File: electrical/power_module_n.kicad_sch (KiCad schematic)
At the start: 16 parts, among them J1 Ground connector from bulb wi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, J10 Need to cut return bulb wiring, J5 Power connector for bulb driv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, Q3 BC548B, Q5 IFRZ44N

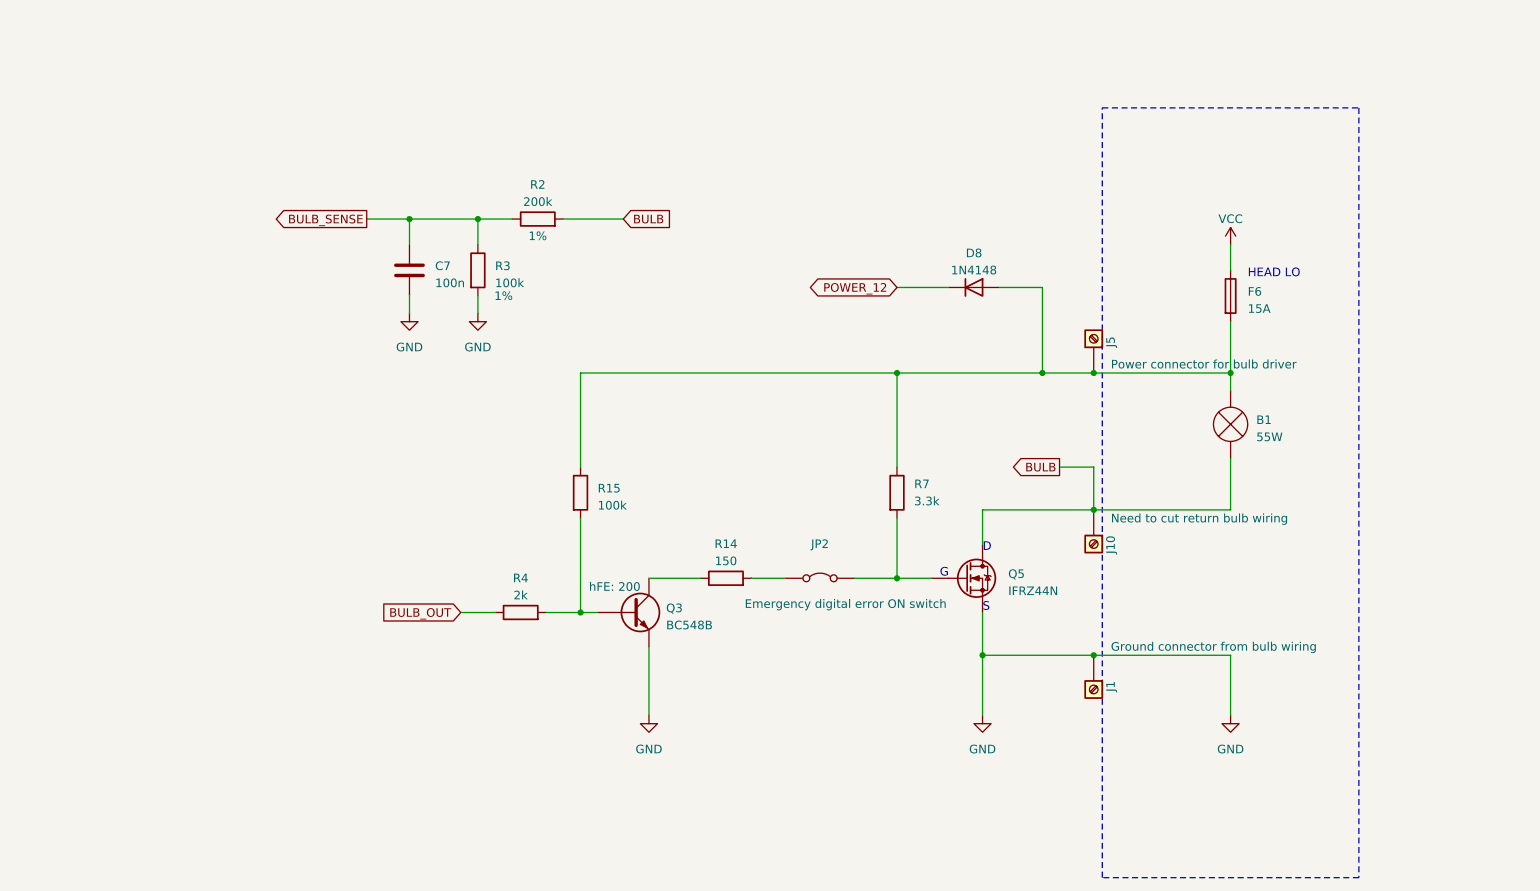
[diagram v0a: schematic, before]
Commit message: Względenie działa
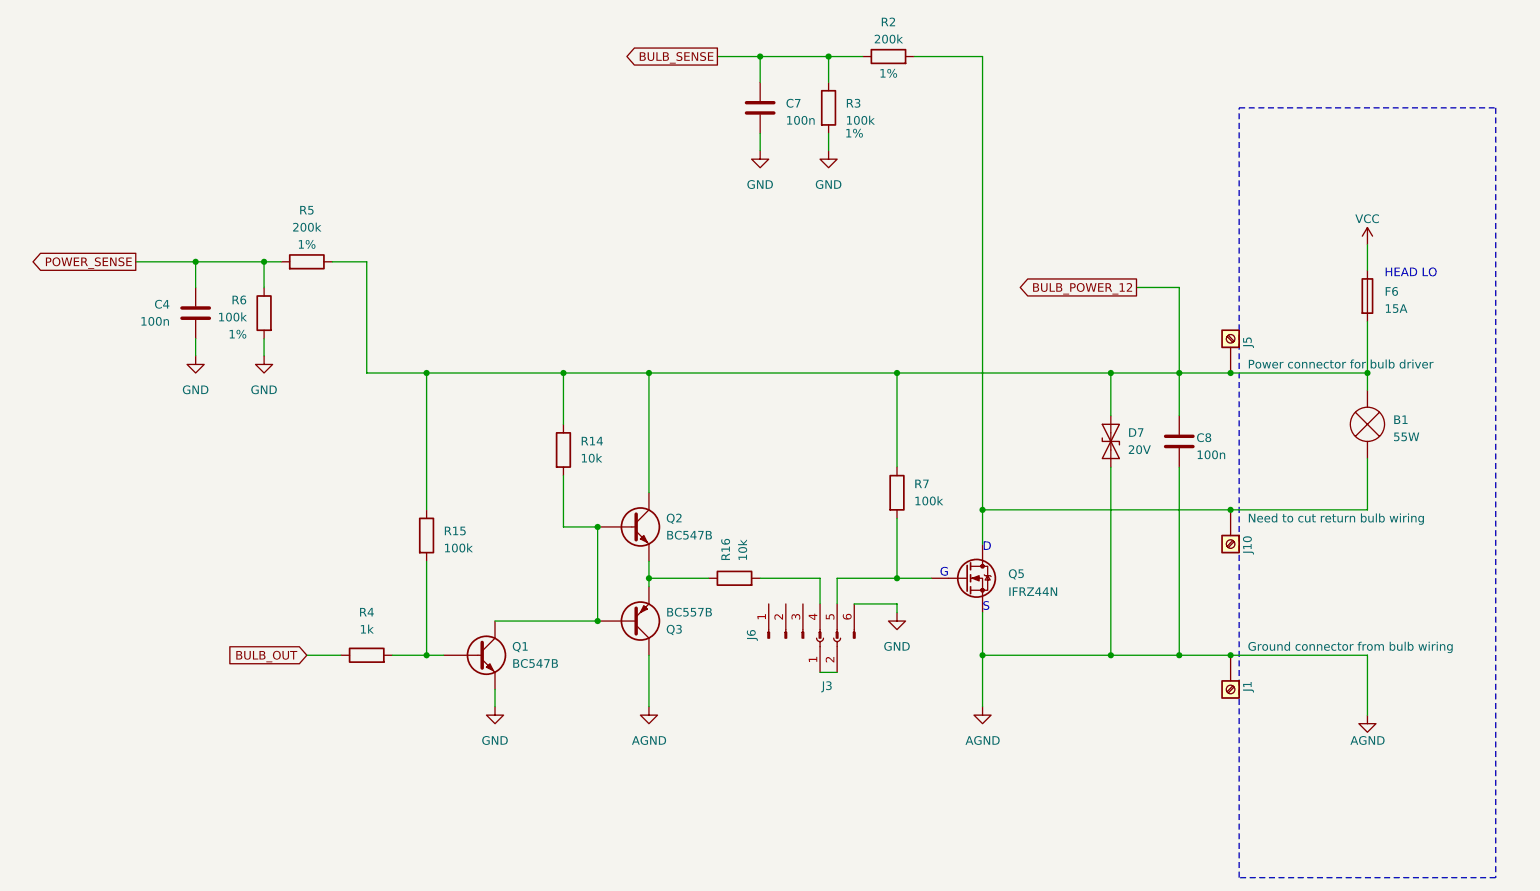
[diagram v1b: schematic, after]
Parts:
- removed D8: 1N4148, Diode_THT:D_DO-41_SOD81_P10.16mm_Horizontal, symbol Diode:1N4002
- removed JP2: Emergency digital error ON switch, symbol Jumper:Jumper_2_Bridged
- removed Q3: BC548B, Package_TO_SOT_THT:TO-92_Inline, symbol Transistor_BJT:BC547
- added C4, C8: 100n, symbol Device:C
- added D7: 20V, symbol Diode:SD05_SOD323
- added J3: Conn_01x02_Socket, symbol Connector:Conn_01x02_Socket
- added J6: Conn_01x06_Pin, symbol Connector:Conn_01x06_Pin
- added Q1, Q2: BC547B, Package_TO_SOT_THT:TO-92_Inline, symbol Transistor_BJT:BC547
- added Q3: BC557B, Package_TO_SOT_THT:TO-92_Inline, symbol Transistor_BJT:BC557
- added R16: 10k, symbol Device:R
- added R5: 200k, symbol Device:R
- added R6: 100k, symbol Device:R
- R14: value 150 -> 10k
- R4: value 2k -> 1k
- R7: value 3.3k -> 100k
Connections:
- net GND: now also C4.2, J6.6 (Pin_6), Q1.3 (E), R6.2; no longer J1.1 (Pin_1), Q5.3 (S)
- net BULB_POWER_12: now reaches B1.2 (+), F6.2, J5.1 (Pin_1), R15.1, R7.1
- net BULB_POWER_12: now also R14.1, C8.1, D7.2 (A2), Q2.1 (C), R5.1
- net at Q5.1 (G), R7.2: now also J6.5 (Pin_5)
- net at R14.2: now also Q1.1 (C), Q2.2 (B), Q3.2 (B)
- net at R15.2, R4.2: now also Q1.2 (B)
- net BULB: no longer names the net of B1.1 (-), J10.1 (Pin_1), Q5.2 (D), R2.2
- new net: Q2.3 (E), Q3.3 (E), R16.1
- new net: J6.4 (Pin_4), R16.2
- new net: J3.1 (Pin_1), J3.2 (Pin_2)
- new net AGND: C8.2, D7.1 (A1), J1.1 (Pin_1), Q3.1 (C), Q5.3 (S)
- new net POWER_SENSE: C4.1, R5.2, R6.1
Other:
- moved on the sheet: B1, C7, F6, J1, J10, J5, R15, R2, R3, R4
